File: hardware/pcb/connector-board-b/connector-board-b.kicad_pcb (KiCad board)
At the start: 2 copper layers, 27.4 x 70.6 mm, 46 parts, among them J1 DE9_Pins, J2 PANEL_18V, J5 8-215570-0, J6 NTC_103AT, J7 BATTERY, Q1 Si4840BDY, Q2 Si4840BDY, SW1 PWR_KILL, U1 BQ24650RVA, U2 INA3221, U3 MCP1700-3.3

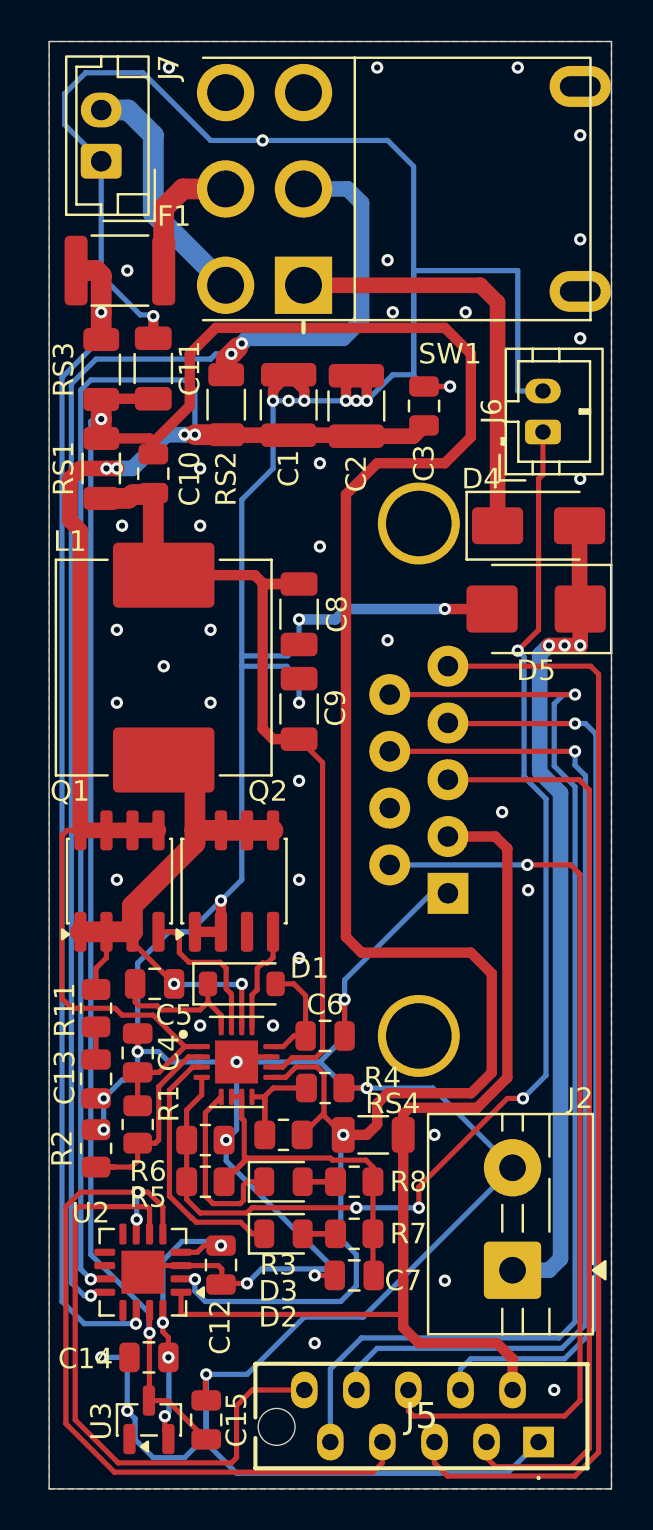
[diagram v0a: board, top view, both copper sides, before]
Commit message: Parts ordered!
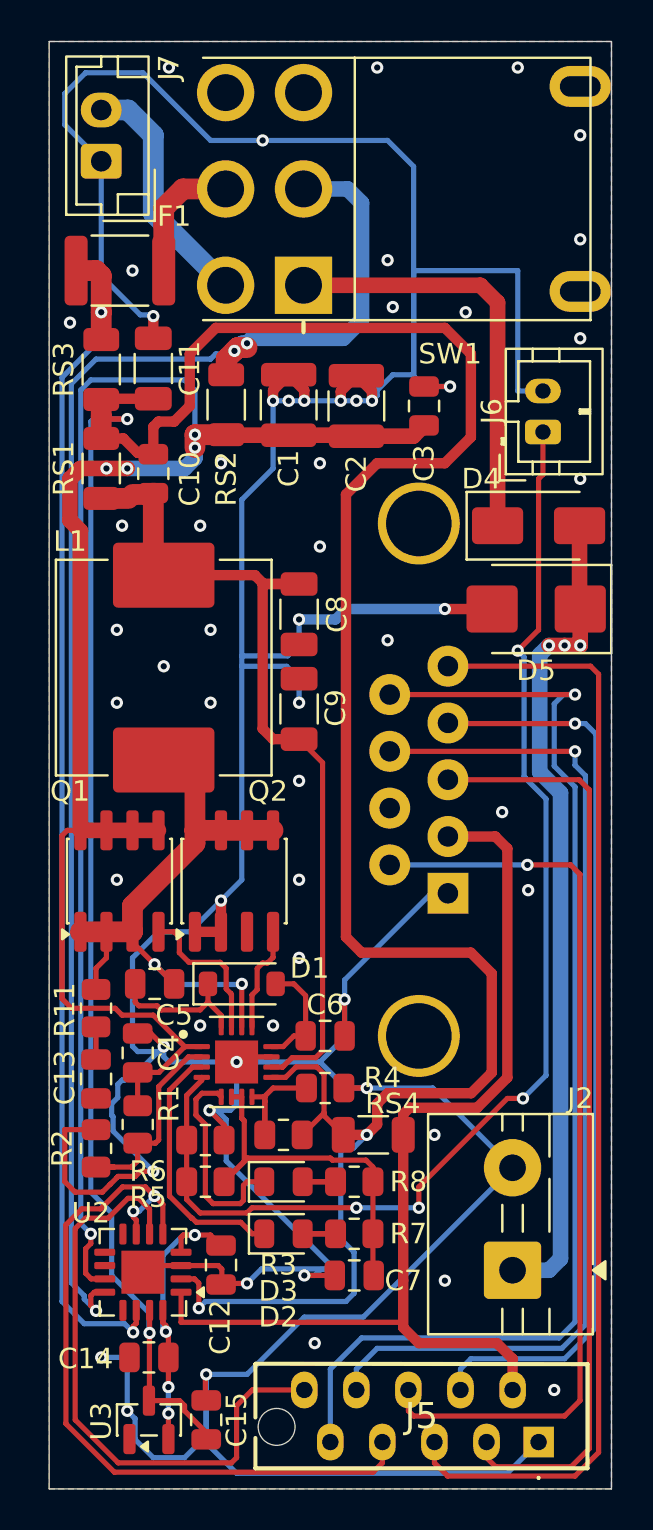
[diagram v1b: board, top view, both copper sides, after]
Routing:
- net GND: track 256.5 -> 275.0 mm
- net VCC: track 161.5 -> 167.0 mm
- net PANEL+: track 71.7 -> 73.8 mm
- net Net-(U1-PH): track 29.5 -> 30.9 mm
- net Net-(D3-K): track 9.06 -> 10.2 mm
- net VIN: track 112.7 -> 113.5 mm
- net VLOAD+: track 51.6 -> 52.4 mm
- net VBAT: track 58.2 -> 58.7 mm
